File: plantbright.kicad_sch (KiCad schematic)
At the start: 21 parts, among them J1 POWER OUT, J2 5V IN, Q1 AO3400A, Q2 AO3400A, Q3 AO3400A, Q5 AO3400A, SW1 USER 0, U1 XIAO-ESP32-C6

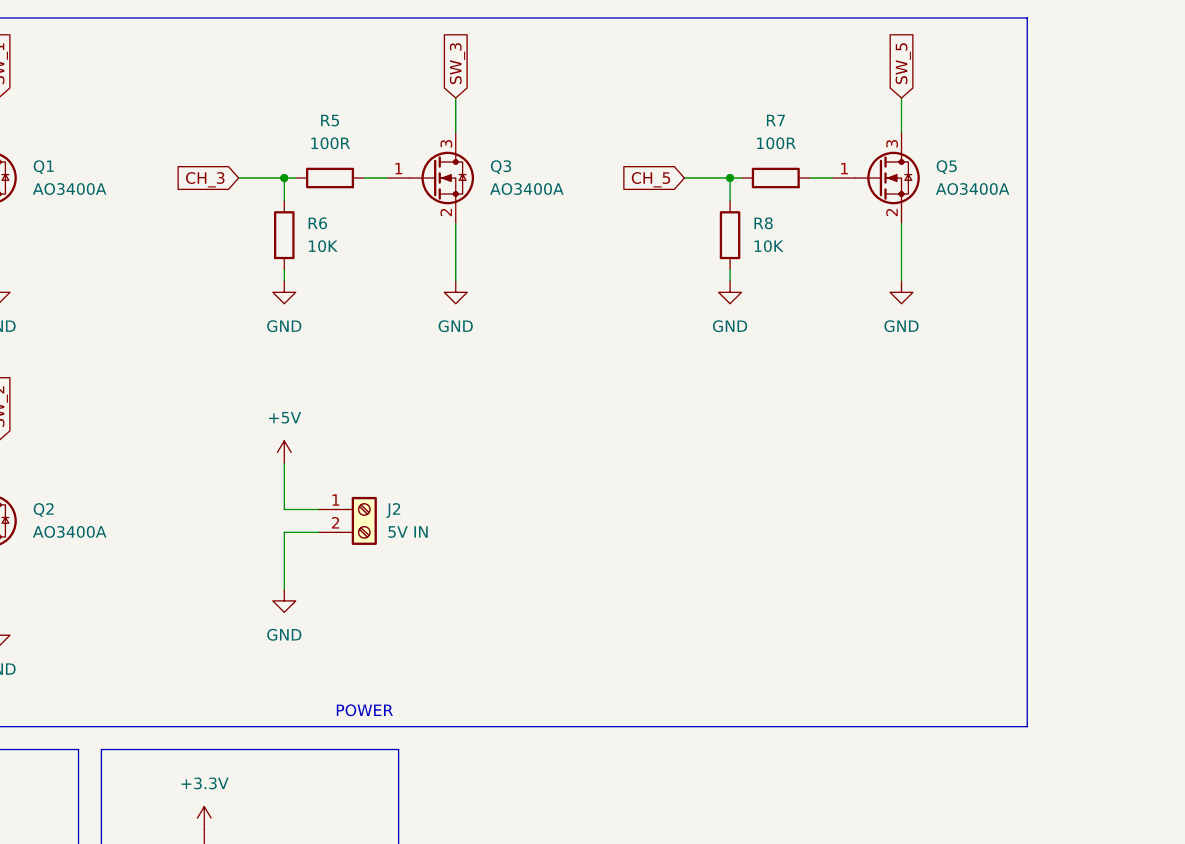
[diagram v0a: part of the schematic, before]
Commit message: Layout 'ings
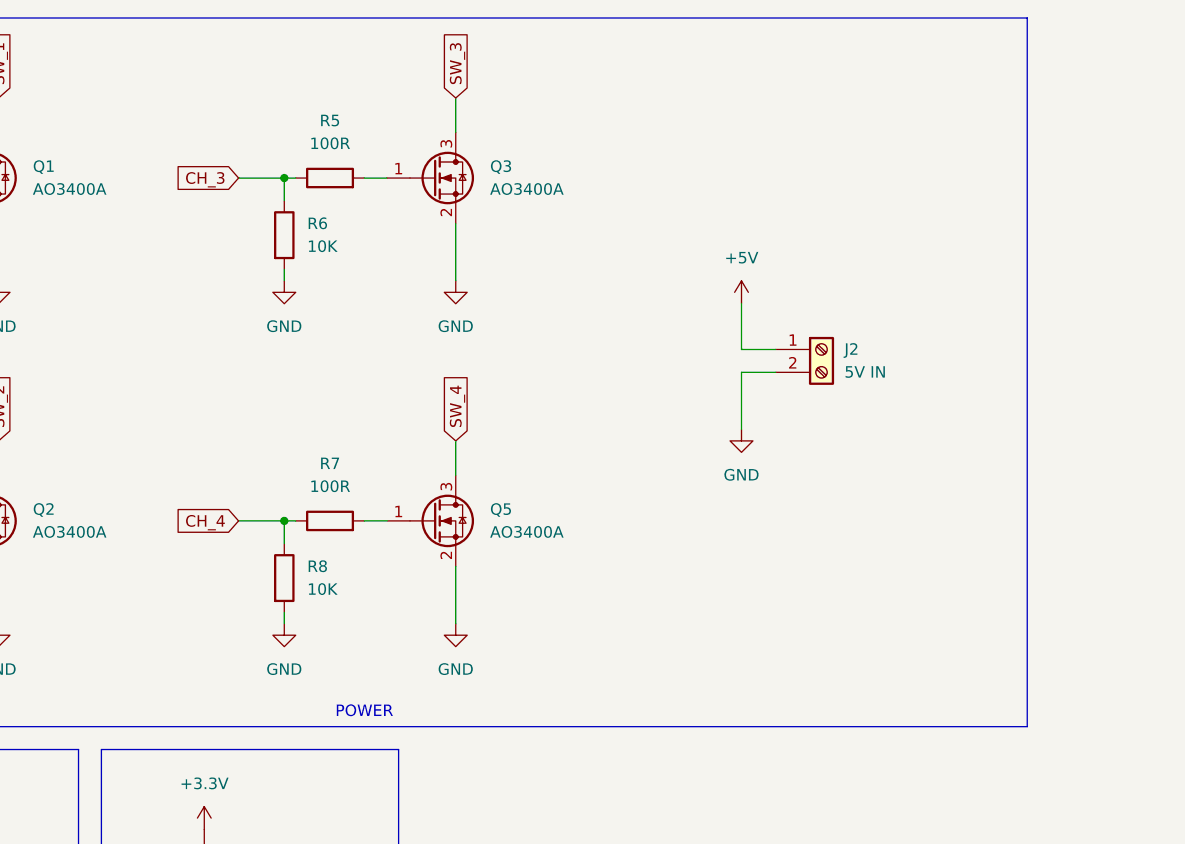
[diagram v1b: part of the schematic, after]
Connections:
- net CH_5 is gone; now on net CH_4: R7.1, R8.1
- net SW_5 is gone; now on net SW_4: Q5.3 (D)
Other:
- moved on the sheet: J2, Q5, R7, R8
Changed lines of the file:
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@@
 	)
 	(junction
-		(at 132.08 35.56)
+		(at 82.55 73.66)
 		(diameter 0)
 		(color 0 0 0 0)
@@
 	(wire
 		(pts
-			(xy 151.13 26.67) (xy 151.13 30.48)
+			(xy 101.6 64.77) (xy 101.6 68.58)
 		)
 		(stroke
@@
 	(wire
 		(pts
-			(xy 82.55 74.93) (xy 86.36 74.93)
+			(xy 133.35 57.15) (xy 137.16 57.15)
 		)
 		(stroke
@@
 	(wire
 		(pts
-			(xy 82.55 72.39) (xy 82.55 67.31)
+			(xy 133.35 54.61) (xy 133.35 49.53)
 		)
 		(stroke
@@
 	(wire
 		(pts
-			(xy 140.97 35.56) (xy 143.51 35.56)
+			(xy 91.44 73.66) (xy 93.98 73.66)
 		)
 		(stroke
@@
 	(wire
 		(pts
-			(xy 82.55 81.28) (xy 82.55 74.93)
+			(xy 133.35 63.5) (xy 133.35 57.15)
 		)
 		(stroke
@@
 	(wire
 		(pts
-			(xy 86.36 72.39) (xy 82.55 72.39)
+			(xy 137.16 54.61) (xy 133.35 54.61)
 		)
 		(stroke
@@
 	(wire
 		(pts
-			(xy 132.08 38.1) (xy 132.08 35.56)
+			(xy 82.55 76.2) (xy 82.55 73.66)
 		)
 		(stroke
@@
 	(wire
 		(pts
-			(xy 151.13 40.64) (xy 151.13 46.99)
+			(xy 101.6 78.74) (xy 101.6 85.09)
 		)
 		(stroke
@@
 	(wire
 		(pts
-			(xy 127 35.56) (xy 132.08 35.56)
+			(xy 77.47 73.66) (xy 82.55 73.66)
 		)
 		(stroke
@@
 	(wire
 		(pts
-			(xy 132.08 45.72) (xy 132.08 46.99)
+			(xy 82.55 83.82) (xy 82.55 85.09)
 		)
 		(stroke
@@
 	(wire
 		(pts
-			(xy 132.08 35.56) (xy 133.35 35.56)
+			(xy 82.55 73.66) (xy 83.82 73.66)
 		)
 		(stroke
@@
 		)
 	)
-	(global_label "CH_5"
+	(global_label "CH_4"
 		(shape input)
-		(at 127 35.56 180)
+		(at 77.47 73.66 180)
 		(fields_autoplaced yes)
 		(effects
@@
 		)
 		(property "Intersheetrefs" "${INTERSHEET_REFS}"
-			(at 119.2372 35.56 0)
+			(at 69.7072 73.66 0)
 			(effects
 				(font
@@
 		)
 	)
-	(global_label "SW_5"
+	(global_label "SW_4"
 		(shape input)
-		(at 151.13 26.67 90)
+		(at 101.6 64.77 90)
 		(fields_autoplaced yes)
 		(effects
@@
 		)
 		(property "Intersheetrefs" "${INTERSHEET_REFS}"
-			(at 151.13 18.8468 90)
+			(at 101.6 56.9468 90)
 			(effects
 				(font
@@
 	(symbol
 		(lib_id "Connector:Screw_Terminal_01x02")
-		(at 91.44 72.39 0)
+		(at 142.24 54.61 0)
 		(unit 1)
 		(exclude_from_sim no)
@@
 		(fields_autoplaced yes)
 		(property "Reference" "J2"
-			(at 93.98 72.3899 0)
+			(at 144.78 54.6099 0)
 			(effects
 				(font
@@
 		)
 		(property "Value" "5V IN"
-			(at 93.98 74.9299 0)
+			(at 144.78 57.1499 0)
 			(effects
 				(font
@@
 		)
 		(property "Footprint" "Connector_JST:JST_XH_B2B-XH-A_1x02_P2.50mm_Vertical"
-			(at 91.44 72.39 0)
+			(at 142.24 54.61 0)
 			(effects
 				(font
@@
 		)
 		(property "Datasheet" "~"
-			(at 91.44 72.39 0)
+			(at 142.24 54.61 0)
 			(effects
 				(font
@@
 		)
 		(property "Description" "Generic screw terminal, single row, 01x02, script generated (kicad-library-utils/schlib/autogen/connector/)"
-			(at 91.44 72.39 0)
+			(at 142.24 54.61 0)
 			(effects
 				(font
@@
 	(symbol
 		(lib_id "Device:R")
-		(at 132.08 41.91 0)
+		(at 82.55 80.01 0)
 		(unit 1)
 		(exclude_from_sim no)
@@
 		(fields_autoplaced yes)
 		(property "Reference" "R8"
-			(at 134.62 40.6399 0)
+			(at 85.09 78.7399 0)
 			(effects
 				(font
@@
 		)
 		(property "Value" "10K"
-			(at 134.62 43.1799 0)
+			(at 85.09 81.2799 0)
 			(effects
 				(font
@@
 		)
 		(property "Footprint" "Resistor_SMD:R_0805_2012Metric_Pad1.20x1.40mm_HandSolder"
-			(at 130.302 41.91 90)
+			(at 80.772 80.01 90)
 			(effects
 				(font
@@
 		)
 		(property "Datasheet" "~"
-			(at 132.08 41.91 0)
+			(at 82.55 80.01 0)
 			(effects
 				(font
@@
 		)
 		(property "Description" "Resistor"
-			(at 132.08 41.91 0)
+			(at 82.55 80.01 0)
 			(effects
 				(font
@@
 	(symbol
 		(lib_id "power:GND")
-		(at 151.13 46.99 0)
+		(at 101.6 85.09 0)
 		(unit 1)
 		(exclude_from_sim no)
@@
 		(fields_autoplaced yes)
 		(property "Reference" "#PWR014"
-			(at 151.13 53.34 0)
+			(at 101.6 91.44 0)
 			(effects
 				(font
@@
 		)
 		(property "Value" "GND"
-			(at 151.13 52.07 0)
+			(at 101.6 90.17 0)
 			(effects
 				(font
@@
 		)
 		(property "Footprint" ""
-			(at 151.13 46.99 0)
+			(at 101.6 85.09 0)
 			(effects
 				(font
@@
 		)
 		(property "Datasheet" ""
-			(at 151.13 46.99 0)
+			(at 101.6 85.09 0)
 			(effects
 				(font
@@
 		)
 		(property "Description" "Power symbol creates a global label with name \"GND\" , ground"
-			(at 151.13 46.99 0)
+			(at 101.6 85.09 0)
 			(effects
 				(font
@@
 	(symbol
 		(lib_id "power:+5V")
-		(at 82.55 67.31 0)
+		(at 133.35 49.53 0)
 		(unit 1)
 		(exclude_from_sim no)
@@
 		(fields_autoplaced yes)
 		(property "Reference" "#PWR020"
-			(at 82.55 71.12 0)
+			(at 133.35 53.34 0)
 			(effects
 				(font
@@
 		)
 		(property "Value" "+5V"
-			(at 82.55 62.23 0)
+			(at 133.35 44.45 0)
 			(effects
 				(font
@@
 		)
 		(property "Footprint" ""
-			(at 82.55 67.31 0)
+			(at 133.35 49.53 0)
 			(effects
 				(font
@@
 		)
 		(property "Datasheet" ""
-			(at 82.55 67.31 0)
+			(at 133.35 49.53 0)
 			(effects
 				(font
@@
 		)
 		(property "Description" "Power symbol creates a global label with name \"+5V\""
-			(at 82.55 67.31 0)
+			(at 133.35 49.53 0)
 			(effects
 				(font
@@
 	(symbol
 		(lib_id "power:GND")
-		(at 132.08 46.99 0)
+		(at 82.55 85.09 0)
 		(unit 1)
 		(exclude_from_sim no)
@@
 		(fields_autoplaced yes)
 		(property "Reference" "#PWR012"
-			(at 132.08 53.34 0)
+			(at 82.55 91.44 0)
 			(effects
 				(font
@@
 		)
 		(property "Value" "GND"
-			(at 132.08 52.07 0)
+			(at 82.55 90.17 0)
 			(effects
 				(font
@@
 		)
 		(property "Footprint" ""
-			(at 132.08 46.99 0)
+			(at 82.55 85.09 0)
 			(effects
 				(font
@@
 		)
 		(property "Datasheet" ""
-			(at 132.08 46.99 0)
+			(at 82.55 85.09 0)
 			(effects
 				(font
@@
 		)
 		(property "Description" "Power symbol creates a global label with name \"GND\" , ground"
-			(at 132.08 46.99 0)
+			(at 82.55 85.09 0)
 			(effects
 				(font
@@
 	(symbol
 		(lib_id "power:GND")
-		(at 82.55 81.28 0)
+		(at 133.35 63.5 0)
 		(unit 1)
 		(exclude_from_sim no)
@@
 		(fields_autoplaced yes)
 		(property "Reference" "#PWR019"
-			(at 82.55 87.63 0)
+			(at 133.35 69.85 0)
 			(effects
 				(font
@@
 		)
 		(property "Value" "GND"
-			(at 82.55 86.36 0)
+			(at 133.35 68.58 0)
 			(effects
 				(font
@@
 		)
 		(property "Footprint" ""
-			(at 82.55 81.28 0)
+			(at 133.35 63.5 0)
 			(effects
 				(font
@@
 		)
 		(property "Datasheet" ""
-			(at 82.55 81.28 0)
+			(at 133.35 63.5 0)
 			(effects
 				(font
@@
 		)
 		(property "Description" "Power symbol creates a global label with name \"GND\" , ground"
-			(at 82.55 81.28 0)
+			(at 133.35 63.5 0)
 			(effects
 				(font
@@
 	(symbol
 		(lib_id "Device:R")
-		(at 137.16 35.56 90)
+		(at 87.63 73.66 90)
 		(unit 1)
 		(exclude_from_sim no)
@@
 		(fields_autoplaced yes)
 		(property "Reference" "R7"
-			(at 137.16 29.21 90)
+			(at 87.63 67.31 90)
 			(effects
 				(font
@@
 		)
 		(property "Value" "100R"
-			(at 137.16 31.75 90)
+			(at 87.63 69.85 90)
 			(effects
 				(font
@@
 		)
 		(property "Footprint" "Resistor_SMD:R_0805_2012Metric_Pad1.20x1.40mm_HandSolder"
-			(at 137.16 37.338 90)
+			(at 87.63 75.438 90)
 			(effects
 				(font
@@
 		)
 		(property "Datasheet" "~"
-			(at 137.16 35.56 0)
+			(at 87.63 73.66 0)
 			(effects
 				(font
@@
 		)
 		(property "Description" "Resistor"
-			(at 137.16 35.56 0)
+			(at 87.63 73.66 0)
 			(effects
 				(font
@@
 	(symbol
 		(lib_id "Transistor_FET:AO3400A")
-		(at 148.59 35.56 0)
+		(at 99.06 73.66 0)
 		(unit 1)
 		(exclude_from_sim no)
@@
 		(fields_autoplaced yes)
 		(property "Reference" "Q5"
-			(at 154.94 34.2899 0)
+			(at 105.41 72.3899 0)
 			(effects
 				(font
@@
 		)
 		(property "Value" "AO3400A"
-			(at 154.94 36.8299 0)
+			(at 105.41 74.9299 0)
 			(effects
 				(font
@@
 		)
 		(property "Footprint" "Package_TO_SOT_SMD:SOT-23"
-			(at 153.67 37.465 0)
+			(at 104.14 75.565 0)
 			(effects
 				(font
@@
 		)
 		(property "Datasheet" "http://www.aosmd.com/pdfs/datasheet/AO3400A.pdf"
-			(at 153.67 39.37 0)
+			(at 104.14 77.47 0)
 			(effects
 				(font
@@
 		)
 		(property "Description" "30V Vds, 5.7A Id, N-Channel MOSFET, SOT-23"
-			(at 148.59 35.56 0)
+			(at 99.06 73.66 0)
 			(effects
 				(font
